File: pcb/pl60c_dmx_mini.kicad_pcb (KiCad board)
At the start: 4 copper layers, 38.5 x 28.5 mm, 35 parts, among them J1 USB-C 16P, J2 XLR-5 female (DMX OUT), Q1 S8050, SW2 BOOT, SW3 USER, U1 ESP32-S3-MINI-1-N8, U2 AP2112K-3.3, U3 SP3485EN, U4 USBLC6-2SC6

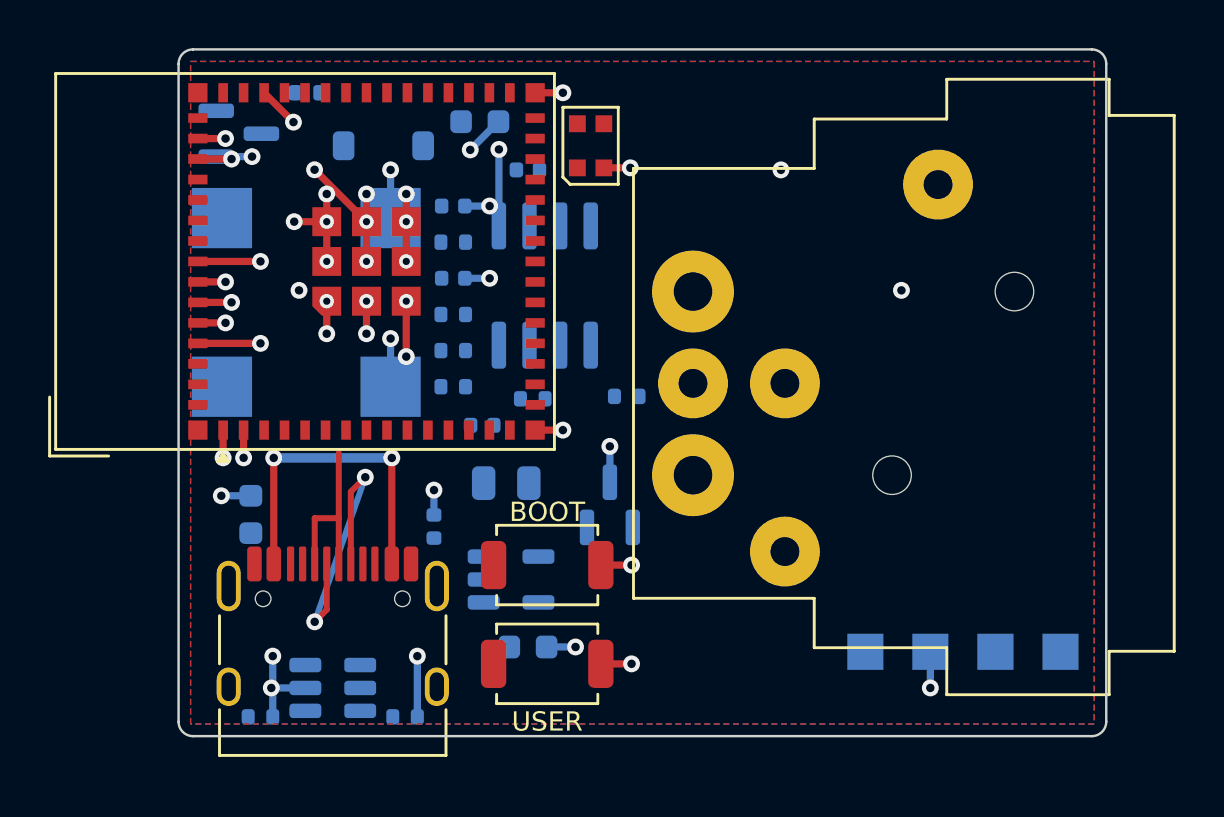
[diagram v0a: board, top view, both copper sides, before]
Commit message: auto: 2026-09-02 14:14:01
Co-Authored-By: Claude Fable 5.1 <noreply@anthropic.com>
Claude-Session: https://claude.ai/code/session_01WsrVZb94LwbHVAmBvsSTfn
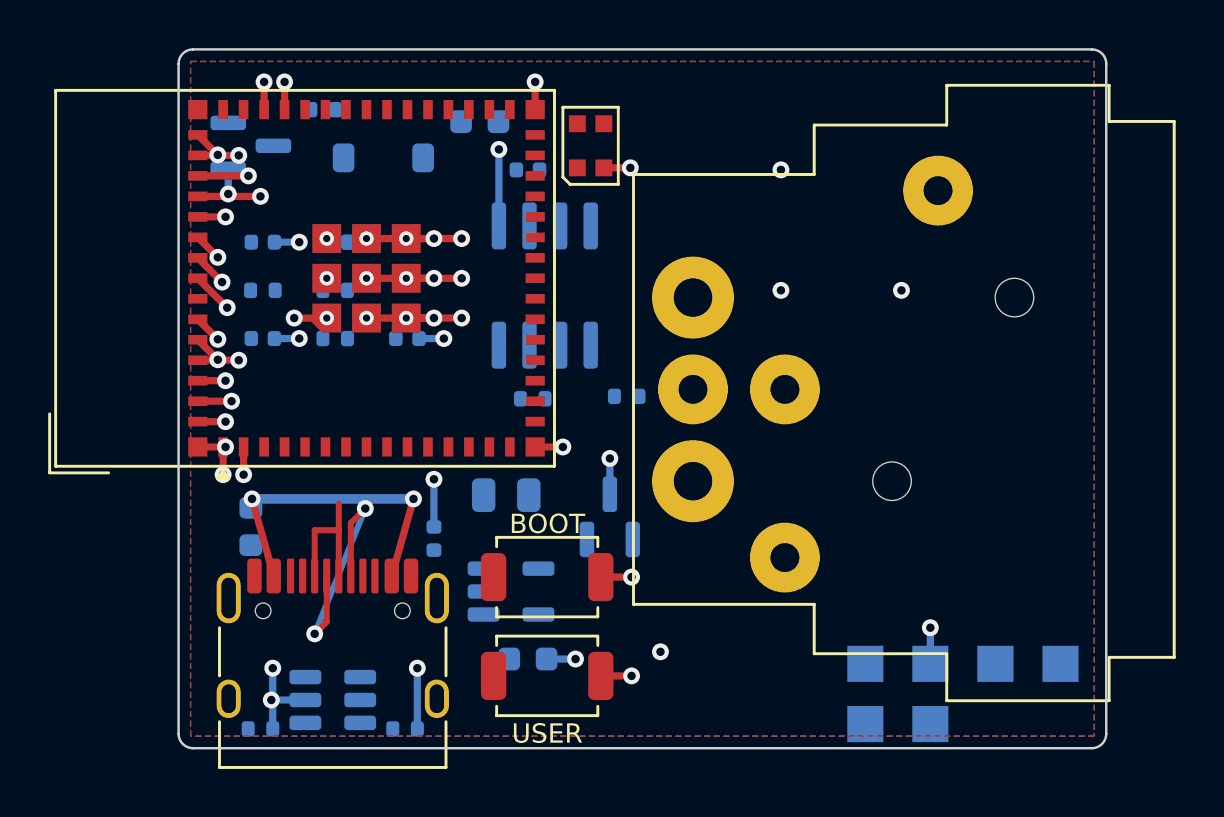
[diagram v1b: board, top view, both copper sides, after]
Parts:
- removed BZ1: MLT-8530, MagneticBuzzer_CUI_CMT-8504-100-SMT
- added TP5: BZ+, TestPoint_Pad_1.5x1.5mm, B.Cu at (28.5, 28.0)
- added TP6: BZ-, TestPoint_Pad_1.5x1.5mm, B.Cu at (31.2, 28.0)
- moved C6 8.29 mm to (3.50, 12.0)
- moved R3 8.15 mm to (3.50, 10.0)
- moved C5 8.04 mm to (3.50, 8.00)
- moved R4 5.75 mm to (6.50, 8.00)
- moved R5 5.50 mm to (6.50, 10.0)
- moved R8 5.29 mm to (6.50, 12.0)
- moved C8 4.75 mm to (9.50, 12.0)
- moved R9 0.96 mm to (6.00, 2.50)
- moved Q1 0.71 mm to (3.00, 4.00)
- moved U1 0.70 mm to (5.25, 9.50)
- moved C1 0.50 mm to (3.00, 19.8)
- moved C2 0.50 mm to (14.5, 25.3)
- moved C3 0.50 mm to (10.6, 20.3)
- moved D1 0.50 mm to (17.9, 19.4)
- moved D3 0.50 mm to (8.50, 4.50)
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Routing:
- net GND: track 64.5 -> 69.1 mm, vias 50 -> 56
- net USB_D-: track 7.50 -> 5.90 mm
- net USB_D+: track 12.8 -> 11.3 mm
- added copper zone on In2.Cu, net GND
- removed copper zone on In2.Cu, net +3V3
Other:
- board size 38.5 x 28.5 mm -> 38.5 x 29 mm
- board text added: "BZ+ BZ-"
